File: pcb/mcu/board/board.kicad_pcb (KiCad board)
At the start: 2 copper layers, 20 parts, among them J1 Conn_02x04_Odd_Even, J2 SCL, J3 SDA, J4 ~RST, J5 PG4, J6 VCC, J7 GND, J8 DTR, Y1 Crystal

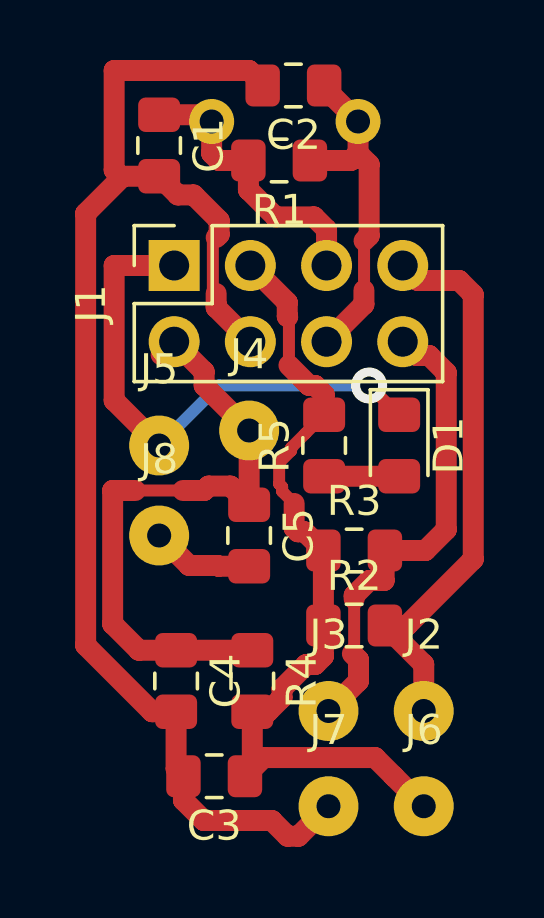
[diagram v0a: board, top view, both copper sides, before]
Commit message: New kicad tested.
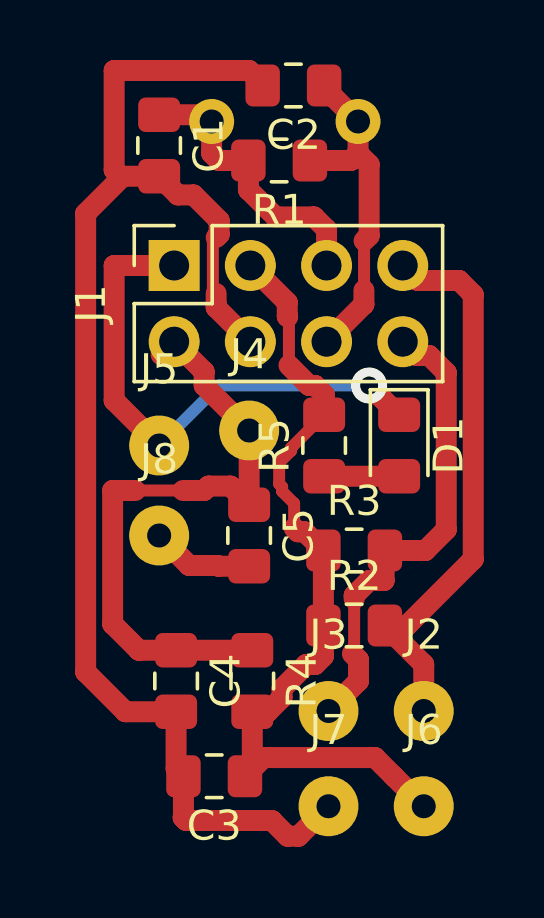
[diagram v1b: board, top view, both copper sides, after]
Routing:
- net GND: track 46.3 -> 47.2 mm
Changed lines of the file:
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@@
-(kicad_pcb (version 20171130) (host pcbnew 5.1.1)
+(kicad_pcb (version 20171130) (host pcbnew 5.1.2)
   (general
     (thickness 1.6)
@@
   )
   (setup
-    (last_trace_width 0.7)
+    (last_trace_width 0.4)
     (user_trace_width 0.4)
     (user_trace_width 0.5)
@@
   (segment (start 76.065 74.28) (end 76.31 74.525) (width 0.7) (layer F.Cu) (net 1))
   (segment (start 76.065 72.375) (end 76.065 74.28) (width 0.7) (layer F.Cu) (net 1))
-  (segment (start 80.145511 76.524489) (end 81.145 75.525) (width 0.7) (layer F.Cu) (net 1))
-  (segment (start 79.780997 76.524489) (end 80.145511 76.524489) (width 0.7) (layer F.Cu) (net 1))
-  (segment (start 79.256508 76) (end 79.780997 76.524489) (width 0.7) (layer F.Cu) (net 1))
-  (segment (start 76.985 76) (end 79.256508 76) (width 0.7) (layer F.Cu) (net 1))
-  (segment (start 76.31 75.325) (end 76.985 76) (width 0.7) (layer F.Cu) (net 1))
-  (segment (start 76.31 74.525) (end 76.31 75.325) (width 0.7) (layer F.Cu) (net 1))
   (segment (start 77.289999 56.677999) (end 77.289999 58.322001) (width 0.4) (layer F.Cu) (net 1))
   (segment (start 77.289999 58.322001) (end 77.400001 58.432003) (width 0.4) (layer F.Cu) (net 1))
   (segment (start 77.5 56.467998) (end 77.289999 56.677999) (width 0.4) (layer F.Cu) (net 1))
-  (segment (start 76.065 72.375) (end 75.265 72.375) (width 0.7) (layer F.Cu) (net 1))
-  (segment (start 73.050498 55.764482) (end 74.24999 54.56499) (width 0.7) (layer F.Cu) (net 1))
-  (segment (start 73.050498 70.160498) (end 73.050498 55.764482) (width 0.7) (layer F.Cu) (net 1))
-  (segment (start 75.265 72.375) (end 73.050498 70.160498) (width 0.7) (layer F.Cu) (net 1))
   (segment (start 74 54.315) (end 74.24999 54.56499) (width 0.7) (layer F.Cu) (net 1))
   (segment (start 74 51) (end 74 54.315) (width 0.7) (layer F.Cu) (net 1))
@@
   (segment (start 75.5 54.525) (end 76.123372 55.148372) (width 0.7) (layer F.Cu) (net 1))
   (segment (start 76.123372 55.148372) (end 76.648372 55.148372) (width 0.7) (layer F.Cu) (net 1))
+  (segment (start 80.145511 76.524489) (end 81.145 75.525) (width 0.7) (layer F.Cu) (net 1))
+  (segment (start 76.31 74.525) (end 76.31 75.89) (width 0.7) (layer F.Cu) (net 1))
+  (segment (start 79.780997 76.524489) (end 80.145511 76.524489) (width 0.7) (layer F.Cu) (net 1))
+  (segment (start 76.31 75.89) (end 76.3 75.9) (width 0.7) (layer F.Cu) (net 1))
+  (segment (start 76.3 75.9) (end 76.4 76) (width 0.7) (layer F.Cu) (net 1))
+  (segment (start 76.4 76) (end 79.256508 76) (width 0.7) (layer F.Cu) (net 1))
+  (segment (start 79.256508 76) (end 79.780997 76.524489) (width 0.7) (layer F.Cu) (net 1))
+  (segment (start 73.050498 55.764482) (end 74.24999 54.56499) (width 0.7) (layer F.Cu) (net 1))
+  (segment (start 73.050498 71.050498) (end 73.050498 55.764482) (width 0.7) (layer F.Cu) (net 1))
+  (segment (start 76.065 72.375) (end 74.375 72.375) (width 0.7) (layer F.Cu) (net 1))
+  (segment (start 74.375 72.375) (end 73.050498 71.050498) (width 0.7) (layer F.Cu) (net 1))
   (segment (start 77.025 52.475) (end 77.25 52.7) (width 0.7) (layer F.Cu) (net 2))
   (segment (start 75.5 52.475) (end 77.025 52.475) (width 0.7) (layer F.Cu) (net 2))
@@
   (segment (start 80.975 67) (end 80.351628 66.376628) (width 0.7) (layer F.Cu) (net 6))
   (segment (start 80.123372 66.376628) (end 80 66.253256) (width 0.7) (layer F.Cu) (net 6))
-  (segment (start 80 66.253256) (end 80 65.431388) (width 0.7) (layer F.Cu) (net 6))
-  (segment (start 80.376628 63.098372) (end 81 62.475) (width 0.4) (layer F.Cu) (net 6))
-  (segment (start 79.899491 63.575509) (end 80.376628 63.098372) (width 0.4) (layer F.Cu) (net 6))
-  (segment (start 79.60001 65.031398) (end 79.60001 64.880754) (width 0.4) (layer F.Cu) (net 6))
-  (segment (start 80 65.431388) (end 79.60001 65.031398) (width 0.4) (layer F.Cu) (net 6))
-  (segment (start 79.5 64.071248) (end 79.899491 63.671757) (width 0.4) (layer F.Cu) (net 6))
-  (segment (start 79.5 64.780744) (end 79.5 64.071248) (width 0.4) (layer F.Cu) (net 6))
-  (segment (start 79.60001 64.880754) (end 79.5 64.780744) (width 0.4) (layer F.Cu) (net 6))
-  (segment (start 79.899491 63.671757) (end 79.899491 63.575509) (width 0.4) (layer F.Cu) (net 6))
   (segment (start 79.77 59.197998) (end 79.786001 59.213999) (width 0.7) (layer F.Cu) (net 6))
   (segment (start 78.54 57.5) (end 79.77 58.73) (width 0.7) (layer F.Cu) (net 6))
@@
   (segment (start 81 62.475) (end 81 61.8) (width 0.7) (layer F.Cu) (net 6))
   (segment (start 81 61.8) (end 80.7 61.5) (width 0.7) (layer F.Cu) (net 6))
+  (segment (start 80 65.431388) (end 80 66.253256) (width 0.4) (layer F.Cu) (net 6))
+  (segment (start 79.60001 65.031398) (end 80 65.431388) (width 0.4) (layer F.Cu) (net 6))
+  (segment (start 79.5 64.780744) (end 79.60001 64.880754) (width 0.4) (layer F.Cu) (net 6))
+  (segment (start 81 62.475) (end 79.899491 63.575509) (width 0.4) (layer F.Cu) (net 6))
+  (segment (start 79.899491 63.671757) (end 79.5 64.071248) (width 0.4) (layer F.Cu) (net 6))
+  (segment (start 79.5 64.071248) (end 79.5 64.780744) (width 0.4) (layer F.Cu) (net 6))
+  (segment (start 79.899491 63.575509) (end 79.899491 63.671757) (width 0.4) (layer F.Cu) (net 6))
+  (segment (start 79.60001 64.880754) (end 79.60001 65.031398) (width 0.4) (layer F.Cu) (net 6))
   (segment (start 75.565 60.475) (end 76 60.04) (width 0.7) (layer F.Cu) (net 7))
   (segment (start 76 60.04) (end 77 61.04) (width 0.7) (layer F.Cu) (net 7))
@@
   (segment (start 82.5 61.5) (end 77.5 61.5) (width 0.4) (layer B.Cu) (net 8))
   (segment (start 77.5 61.5) (end 75.5 63.5) (width 0.4) (layer B.Cu) (net 8))
-  (segment (start 83.475 62.475) (end 82.5 61.5) (width 0.4) (layer F.Cu) (net 8))
-  (segment (start 83.5 62.475) (end 83.475 62.475) (width 0.4) (layer F.Cu) (net 8))
   (via (at 82.5 61.5) (size 1.2) (drill 0.6) (layers F.Cu B.Cu) (net 8))
   (segment (start 74 62) (end 75.5 63.5) (width 0.7) (layer F.Cu) (net 8))
   (segment (start 76 57.5) (end 74 57.5) (width 0.7) (layer F.Cu) (net 8))
   (segment (start 74 57.5) (end 74 62) (width 0.7) (layer F.Cu) (net 8))
+  (segment (start 83.475 62.475) (end 82.5 61.5) (width 0.7) (layer F.Cu) (net 8))
+  (segment (start 83.5 62.475) (end 83.475 62.475) (width 0.7) (layer F.Cu) (net 8))
   (segment (start 81 64.525) (end 83.5 64.525) (width 0.7) (layer F.Cu) (net 9))
   (segment (start 77.475 67.525) (end 78.5 67.525) (width 0.7) (layer F.Cu) (net 10))
